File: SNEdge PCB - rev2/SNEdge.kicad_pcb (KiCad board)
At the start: 2 copper layers, 53 x 16.4 mm, 33 parts, among them J10 R_O, J2 R_E, J3 B_E, J4 G_E, J5 G_IN, J6 B_IN, J7 R_IN, J8 G_O, J9 B_O, U1 THS7376

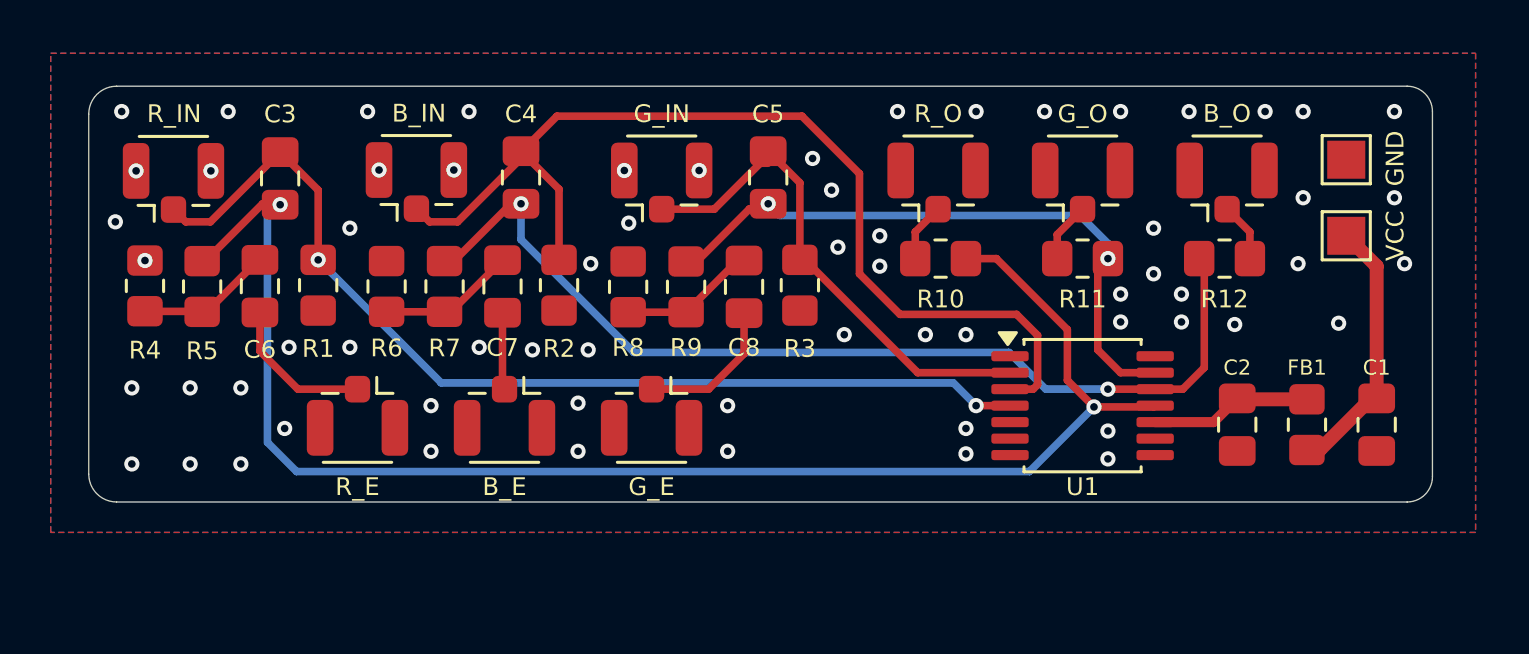
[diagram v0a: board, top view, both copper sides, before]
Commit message: Refactor for purity
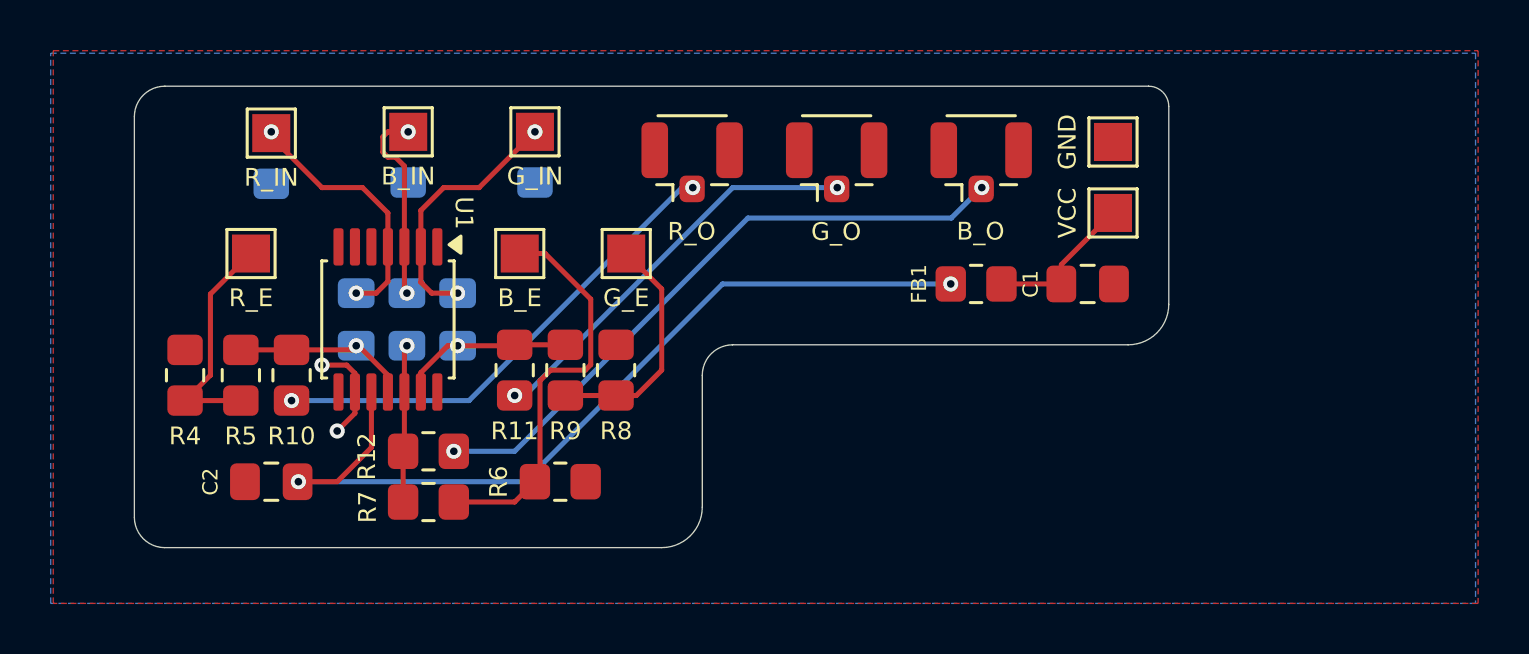
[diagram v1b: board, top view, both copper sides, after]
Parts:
- removed C6, C7, C8: 100nF, Capacitor_SMD:C_0805_2012Metric_Pad1.18x1.45mm_HandSolder
- removed J2: R_E, Connector_Coaxial:U.FL_Hirose_U.FL-R-SMT-1_Vertical
- removed J3: B_E, Connector_Coaxial:U.FL_Hirose_U.FL-R-SMT-1_Vertical
- removed J4: G_E, Connector_Coaxial:U.FL_Hirose_U.FL-R-SMT-1_Vertical
- removed J5: G_IN, Connector_Coaxial:U.FL_Hirose_U.FL-R-SMT-1_Vertical
- removed J6: B_IN, Connector_Coaxial:U.FL_Hirose_U.FL-R-SMT-1_Vertical
- removed J7: R_IN, Connector_Coaxial:U.FL_Hirose_U.FL-R-SMT-1_Vertical
- added TP3: G_IN, TestPoint:TestPoint_Pad_1.5x1.5mm, F.Cu at (121.8, 92.2)
- added TP4: B_IN, TestPoint:TestPoint_Pad_1.5x1.5mm, F.Cu at (116.8, 92.2)
- added TP5: R_IN, TestPoint:TestPoint_Pad_1.5x1.5mm, F.Cu at (111.4, 92.2)
- added TP6: R_E, TestPoint:TestPoint_Pad_1.5x1.5mm, F.Cu at (110.6, 97.0)
- added TP7: B_E, TestPoint:TestPoint_Pad_1.5x1.5mm, F.Cu at (121.2, 97.0)
- added TP8: G_E, TestPoint:TestPoint_Pad_1.5x1.5mm, F.Cu at (125.4, 97.0)
- C3, C4, C5, R1, R2, R3: moved to B.Cu
- R4, R6, R8: value 180R -> 75R
- R5, R7, R9: value 1k -> 430R
- moved C2 38.2 mm to (111.4, 106.0), turned to 0 degrees
- moved R12 32.3 mm to (117.6, 104.8)
- moved U1 27.6 mm to (116.0, 99.6), turned to -90 degrees
- moved R10 26.0 mm to (112.2, 101.8), turned to 90 degrees
- moved R11 22.8 mm to (121.0, 101.6), turned to 90 degrees
- moved FB1 14.2 mm to (139.2, 98.2), turned to 0 degrees
- moved C5 13.5 mm to (118.8, 99.6)
- moved C1 12.7 mm to (143.6, 98.2), turned to 180 degrees
- moved R3 11.6 mm to (121.8, 93.2)
- moved R6 10.3 mm to (122.8, 106.0), turned to 0 degrees
- moved J8 9.73 mm to (133.7, 93.4)
- moved J10 9.73 mm to (128.0, 93.4)
- moved J9 9.73 mm to (139.4, 93.4)
- moved TP1 9.24 mm to (144.6, 95.4)
- moved TP2 9.23 mm to (144.6, 92.6)
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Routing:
- net Net-(U1-CH4_OUT): track 58.9 -> 7.01 mm, vias 2 -> 1
- net Net-(U1-CH3_OUT): track 39.6 -> 6.22 mm, vias 2 -> 1
- net Net-(U1-CH3_IN): track 40.5 -> 7.85 mm, vias 0 -> 2
- net Net-(U1-CH4_IN): track 40.1 -> 10.1 mm
- net VCC: track 6.34 -> 34.6 mm, vias 0 -> 2
- net Net-(J9-In): track 2.42 -> 25.2 mm, vias 0 -> 2
- net Net-(U1-CH2_OUT): track 25.2 -> 6.92 mm, vias 2 -> 1
- net Net-(J10-In): track 2.42 -> 19.5 mm, vias 0 -> 2
- net Net-(J8-In): track 2.36 -> 16.1 mm, vias 0 -> 2
- net Net-(R6-Pad1): track 5.42 -> 16.0 mm
- net Net-(U1-CH2_IN): track 19.8 -> 10.3 mm, vias 0 -> 2
- net Net-(J2-In): track 5.99 -> 0.00 mm
- net Net-(J4-In): track 5.83 -> 0.00 mm
- net Net-(C1-Pad2): track 10.5 -> 6.01 mm
- net GND: track 0.00 -> 4.00 mm, vias 65 -> 2
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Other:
- board size 53 x 16.4 mm -> 40.8 x 18.2 mm
